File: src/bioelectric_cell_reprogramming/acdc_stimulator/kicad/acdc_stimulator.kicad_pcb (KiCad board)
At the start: 4 copper layers, 139 x 133 mm, 144 parts, among them IC1 AD9833BRM-REEL7, IC2 AD5122BCPZ10-RL7, IC3 LTC3896EFE#PBF, IC4 LTC3637IMSE#PBF, IC5 LTC3637IMSE#PBF, IC6 LTC3637IMSE#PBF, J1 Screw_Terminal_01x02, J2 Conn_ARM_SWD_TagConnect_TC203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, J3 USB_C_Receptacle_USB2.0_14P, J4 S4B-PH-SM4-TB, J5 IPL1-102-01-L-S-K, J6 Screw_Terminal_01x02, J7 IPL1-102-01-L-S-K, J8 6620XX11122_66200211122, J9 6620XX11122_66200211122, Q1 BSZ096N10LS5ATMA1, Q10 BSZ096N10LS5ATMA1, Q11 BSZ096N10LS5ATMA1, Q2 NDT3055L, Q3 BSC520N15NS3G, Q4 BSC520N15NS3G, Q5 IPD320N20N3GATMA1, Q6 BSZ096N10LS5ATMA1, Q7 BSZ096N10LS5ATMA1, Q8 IPB320P10LMATMA1, Q9 IPB320P10LMATMA1, SW1 SW_Push, SW2 SW_SPDT, U1 STM32G473RCTx, U2 AMS1117-3.3, U3 USBLC6-2SC6, U4 LTC6090CFE-PBF, U5 LTC6090CFE-PBF, U7 DRV8873HPWPR, Y1 16Mhz

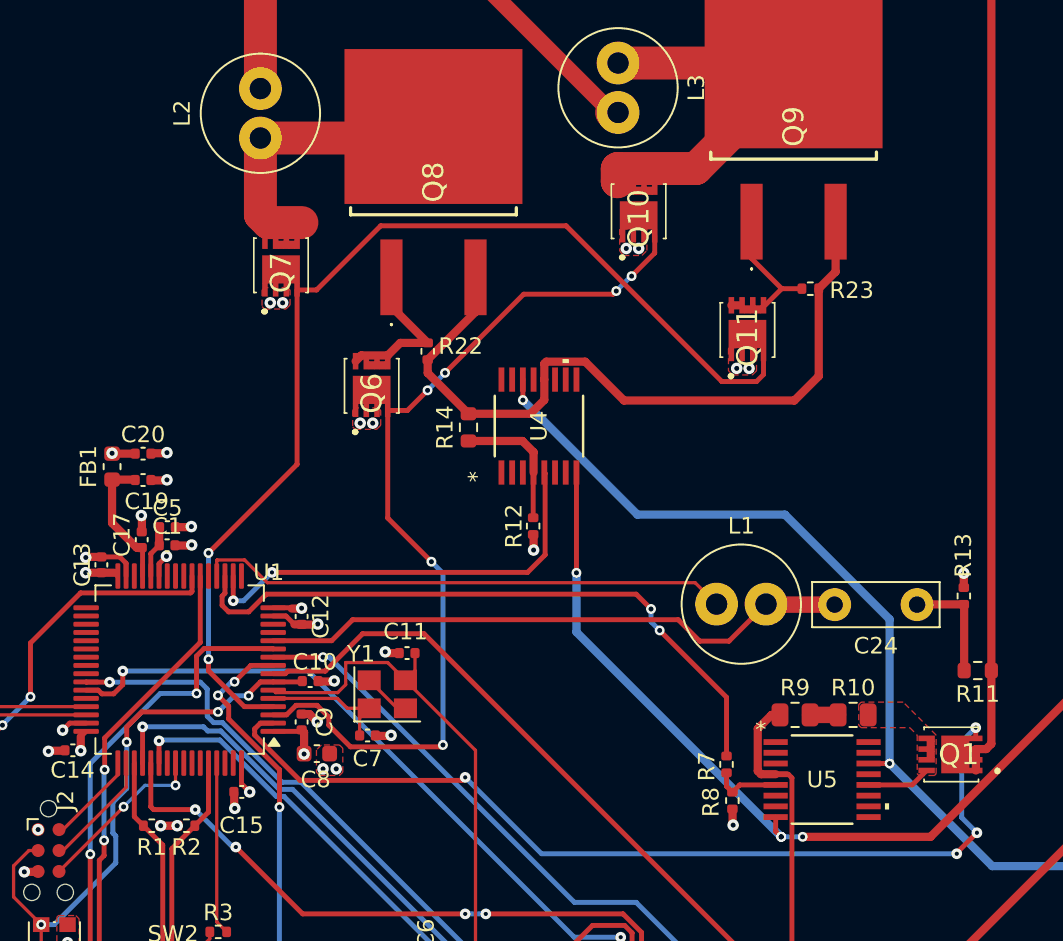
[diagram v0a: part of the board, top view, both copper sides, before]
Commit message: ci: v1 routing complete
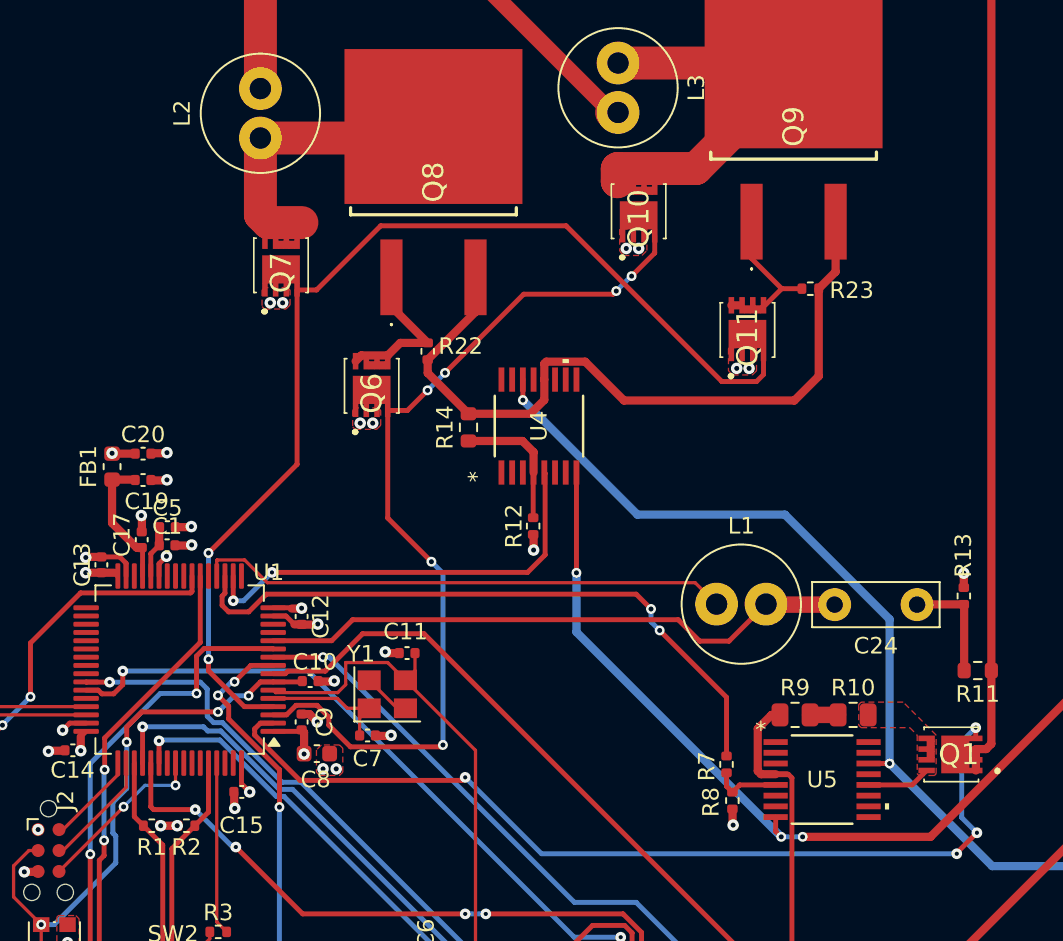
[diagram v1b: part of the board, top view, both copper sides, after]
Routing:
- net Net-(J6-Pin_2): track 52.7 -> 52.0 mm
- net -60V: vias 10 -> 9
